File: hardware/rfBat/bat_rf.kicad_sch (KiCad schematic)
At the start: 89 parts, among them J1 USB_C_Receptacle_PowerOnly_6P, J2 Conn_01x01_Pin, J3 Conn_01x06, J4 Conn_01x03, J5 Conn_01x01_Pin, Q1 NPN, Q3 AO4407, Q5 AllPower__AP2300, SW1 3*4*2.5MM_贴片4脚, SW3 TS-1199A-B-B, U1 ESP32-C3-WROOM-02-N4, U2 IP2325_5M_WHJC, U3 MT2492, U5 MLT-8530-5V, U7 XC6220B331MR

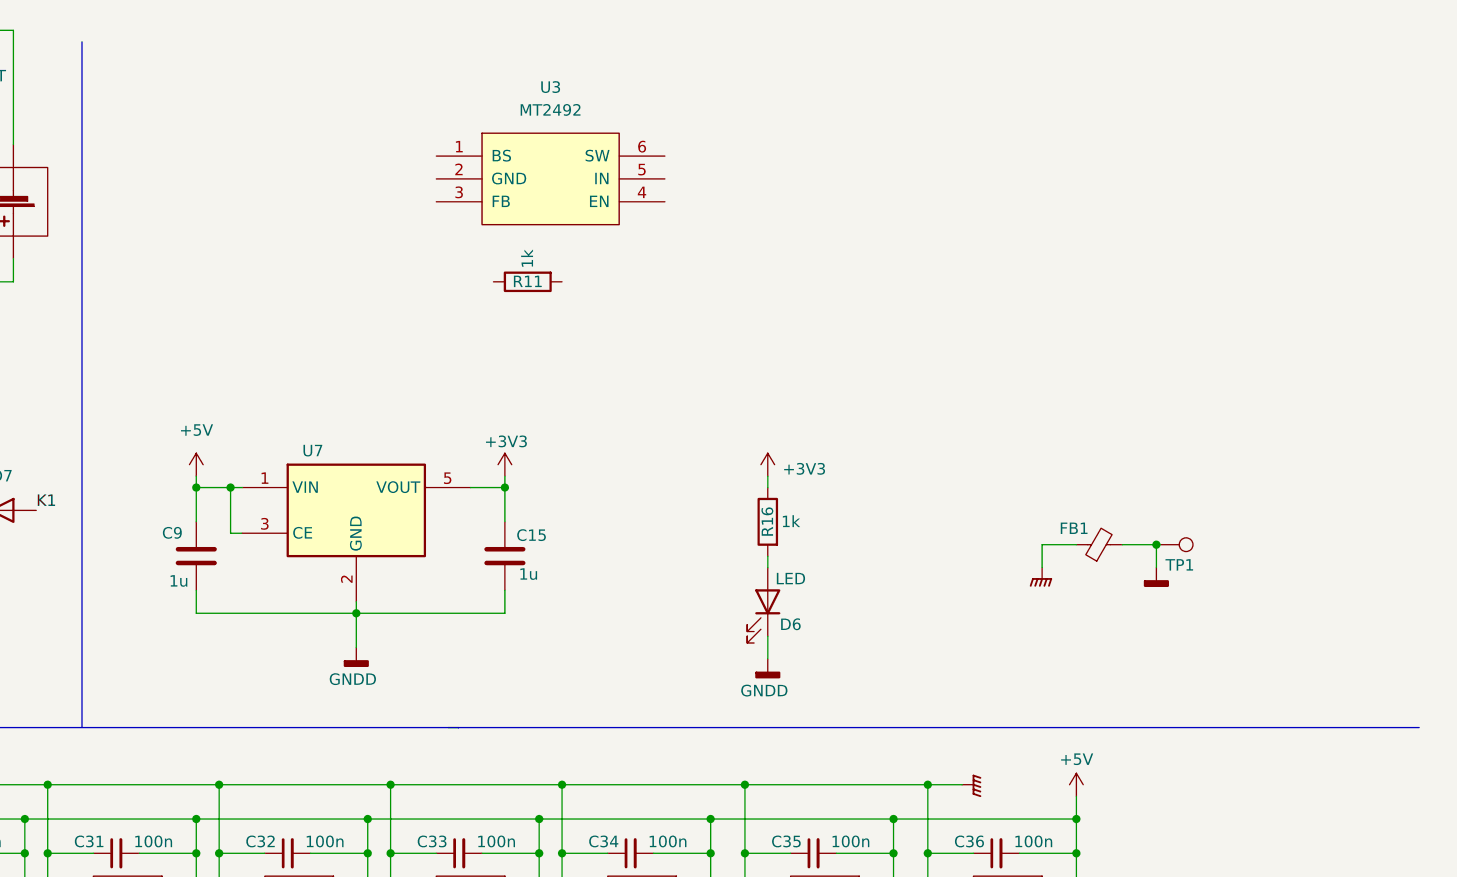
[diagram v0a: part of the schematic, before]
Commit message: update pcb
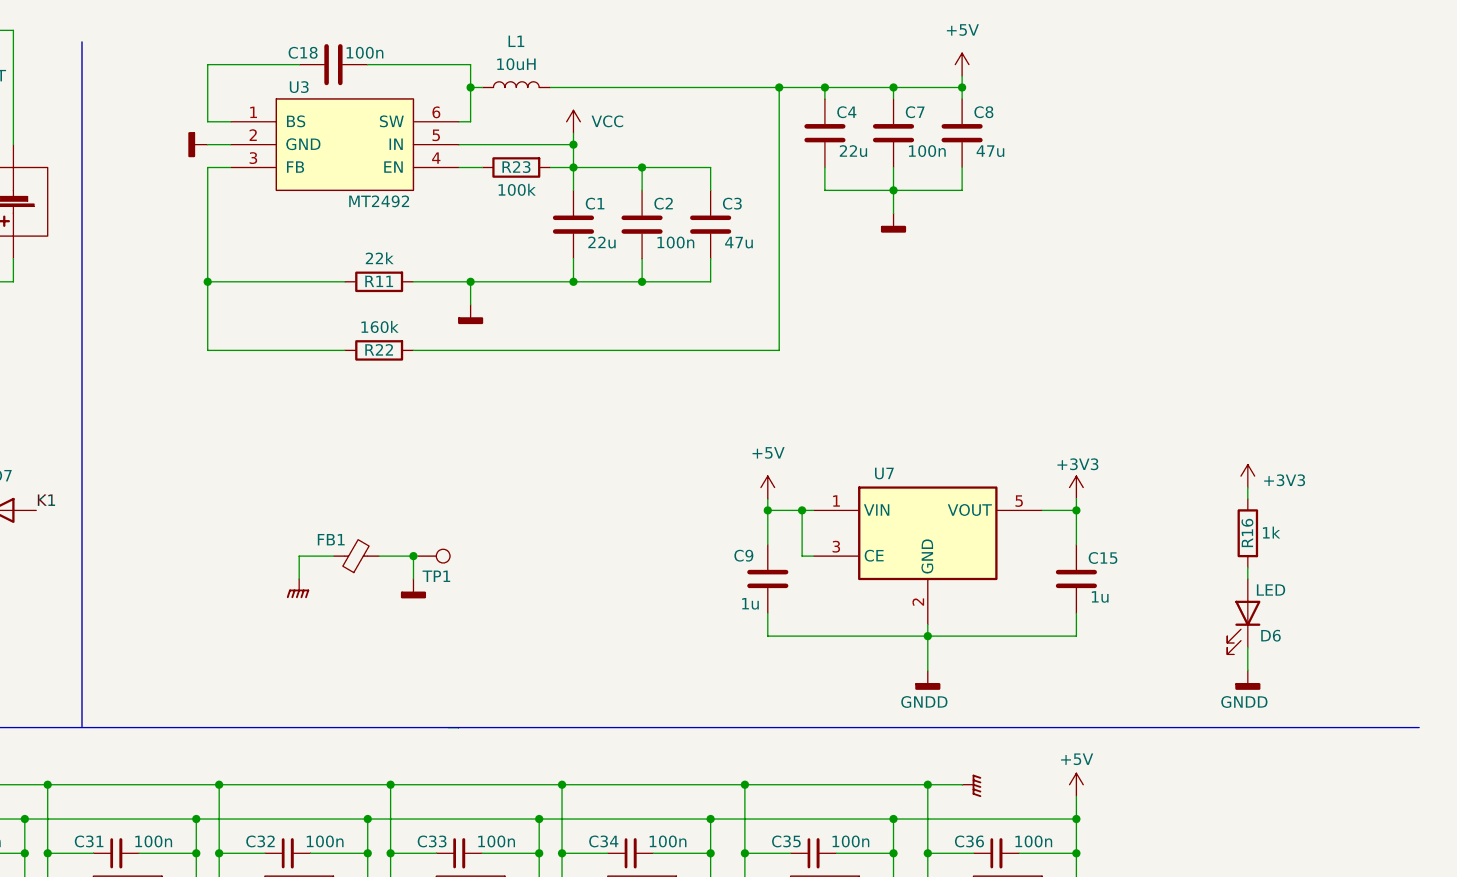
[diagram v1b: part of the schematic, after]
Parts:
- added C1, C4: 22u, Capacitor_SMD:C_0603_1608Metric_Pad1.08x0.95mm_HandSolder, symbol Device:C
- added C18, C2, C7: 100n, Capacitor_SMD:C_0603_1608Metric_Pad1.08x0.95mm_HandSolder, symbol Device:C
- added C3, C8: 47u, Capacitor_SMD:C_0603_1608Metric_Pad1.08x0.95mm_HandSolder, symbol Device:C
- added L1: 10uH, symbol Device:L
- added R22: 160k, Resistor_SMD:R_0603_1608Metric_Pad0.98x0.95mm_HandSolder, symbol Device:R
- added R23: 100k, Resistor_SMD:R_0603_1608Metric_Pad0.98x0.95mm_HandSolder, symbol Device:R
- R11: value 1k -> 22k
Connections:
- net +5V: now also C4.1, C7.1, C8.1, L1.2, R22.2
- net GNDD: now also R11.2, U3.2 (GND), C1.2, C2.2, C3.2, C4.2, C7.2, C8.2
- net VCC: now also U3.5 (IN), C1.1, C2.1, C3.1, R23.2
- net at R11.1: now also U3.3 (FB), R22.1
- net at U3.1 (BS): now also C18.1
- net at U3.4 (EN): now also R23.1
- net at U3.6 (SW): now also C18.2, L1.1
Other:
- moved on the sheet: C15, C9, D6, FB1, R11, R16, TP1, U3, U7
